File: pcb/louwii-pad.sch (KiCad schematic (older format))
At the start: 50 parts, among them J1 USB_B_Micro, J2 ICSP, J3 IIC, K1 KEYSW, K2 KEYSW, K3 KEYSW, K4 KEYSW, K5 KEYSW, K6 KEYSW, K7 KEYSW, K8 KEYSW, SW1 SW_Push, SW6 Rotary_Encoder_Switch, U1 ATmega32U4-atmel, X1 Crystal

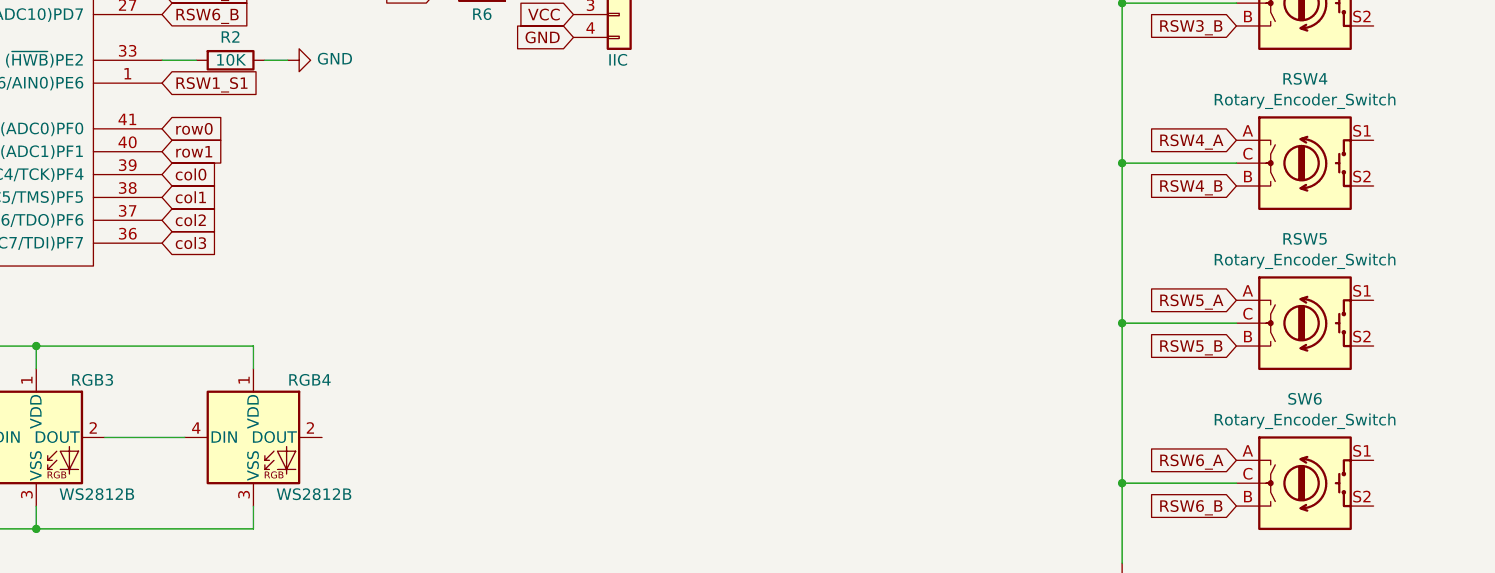
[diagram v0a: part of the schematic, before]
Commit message: finish up schematics and start PCB design
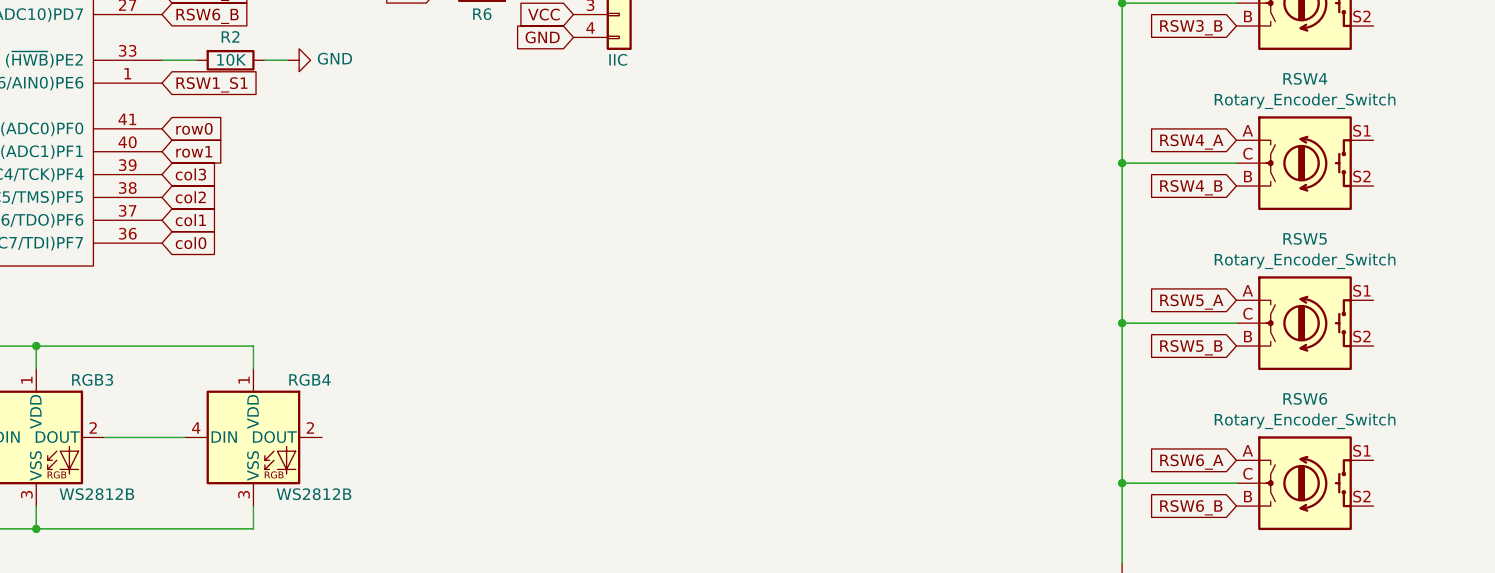
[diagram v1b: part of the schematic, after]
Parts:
- D1, D2, D3, D4, D5, D6, D7, D8: footprint (none) -> Diode_THT:D_DO-35_SOD27_P7.62mm_Horizontal
- J1: footprint (none) -> Connector_USB:USB_Micro-B_Wuerth_629105150521
- J2: footprint (none) -> Connector_PinHeader_2.54mm:PinHeader_2x03_P2.54mm_Vertical
- J3: footprint (none) -> Connector_PinHeader_2.54mm:PinHeader_1x04_P2.54mm_Vertical
- K1, K2, K3, K4, K5, K6, K7, K8: footprint (none) -> Louwii-pad:MX_PCB_100H
- R1, R2, R3, R4, R5, R6: footprint (none) -> Resistor_THT:R_Axial_DIN0207_L6.3mm_D2.5mm_P10.16mm_Horizontal
- RSW1, RSW2, RSW3, RSW4, RSW5: footprint (none) -> Rotary_Encoder:RotaryEncoder_Alps_EC11E-Switch_Vertical_H20mm
- RSW6: renamed from SW6; footprint (none) -> Rotary_Encoder:RotaryEncoder_Alps_EC11E-Switch_Vertical_H20mm
- U1: footprint (none) -> Package_QFP:TQFP-44_10x10mm_P0.8mm
- X1: footprint (none) -> Crystal:Crystal_HC49-U_Vertical
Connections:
- net col0: now also U1.36 ((ADC7/TDI)PF7); no longer U1.39 ((ADC4/TCK)PF4)
- net col1: now also U1.37 ((ADC6/TDO)PF6); no longer U1.38 ((ADC5/TMS)PF5)
- net col2: now also U1.38 ((ADC5/TMS)PF5); no longer U1.37 ((ADC6/TDO)PF6)
- net col3: now also U1.39 ((ADC4/TCK)PF4); no longer U1.36 ((ADC7/TDI)PF7)
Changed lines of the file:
@@
 F 0 "X1" V 1850 3600 50  0000 L CNN
 F 1 "Crystal" V 2250 3500 50  0000 L CNN
-F 2 "" H 2050 3650 50  0001 C CNN
+F 2 "Crystal:Crystal_HC49-U_Vertical" H 2050 3650 50  0001 C CNN
 F 3 "~" H 2050 3650 50  0001 C CNN
 	1    2050 3650
@@
 F 0 "J1" H 7457 1667 50  0000 C CNN
 F 1 "USB_B_Micro" H 7457 1576 50  0000 C CNN
-F 2 "" H 7550 1150 50  0001 C CNN
+F 2 "Connector_USB:USB_Micro-B_Wuerth_629105150521" H 7550 1150 50  0001 C CNN
 F 3 "~" H 7550 1150 50  0001 C CNN
 	1    7400 1200
@@
 F 0 "R3" V 7900 1200 50  0000 C CNN
 F 1 "22" V 8000 1200 50  0000 C CNN
-F 2 "" V 7930 1200 50  0001 C CNN
+F 2 "Resistor_THT:R_Axial_DIN0207_L6.3mm_D2.5mm_P10.16mm_Horizontal" V 7930 1200 50  0001 C CNN
 F 3 "~" H 8000 1200 50  0001 C CNN
 	1    8000 1200
@@
 F 0 "R4" V 8100 1300 50  0000 C CNN
 F 1 "22" V 8000 1300 50  0000 C CNN
-F 2 "" V 7930 1300 50  0001 C CNN
+F 2 "Resistor_THT:R_Axial_DIN0207_L6.3mm_D2.5mm_P10.16mm_Horizontal" V 7930 1300 50  0001 C CNN
 F 3 "~" H 8000 1300 50  0001 C CNN
 	1    8000 1300
@@
 F 0 "R2" V 5250 3600 50  0000 C CNN
 F 1 "10K" V 5350 3600 50  0000 C CNN
-F 2 "" V 5280 3600 50  0001 C CNN
+F 2 "Resistor_THT:R_Axial_DIN0207_L6.3mm_D2.5mm_P10.16mm_Horizontal" V 5280 3600 50  0001 C CNN
 F 3 "~" H 5350 3600 50  0001 C CNN
 	1    5350 3600
@@
 F 0 "R1" V 1900 3200 50  0000 R CNN
 F 1 "10K" V 2000 3300 50  0000 R CNN
-F 2 "" V 1930 3200 50  0001 C CNN
+F 2 "Resistor_THT:R_Axial_DIN0207_L6.3mm_D2.5mm_P10.16mm_Horizontal" V 1930 3200 50  0001 C CNN
 F 3 "~" H 2000 3200 50  0001 C CNN
 	1    2000 3200
@@
 F 0 "RSW1" H 10050 2317 50  0000 C CNN
 F 1 "Rotary_Encoder_Switch" H 10050 2226 50  0000 C CNN
-F 2 "" H 9900 2110 50  0001 C CNN
+F 2 "Rotary_Encoder:RotaryEncoder_Alps_EC11E-Switch_Vertical_H20mm" H 9900 2110 50  0001 C CNN
 F 3 "~" H 10050 2210 50  0001 C CNN
 	1    10050 1950
@@
 F 0 "RSW2" H 10050 3017 50  0000 C CNN
 F 1 "Rotary_Encoder_Switch" H 10050 2926 50  0000 C CNN
-F 2 "" H 9900 2810 50  0001 C CNN
+F 2 "Rotary_Encoder:RotaryEncoder_Alps_EC11E-Switch_Vertical_H20mm" H 9900 2810 50  0001 C CNN
 F 3 "~" H 10050 2910 50  0001 C CNN
 	1    10050 2650
@@
 F 0 "RSW3" H 10050 3717 50  0000 C CNN
 F 1 "Rotary_Encoder_Switch" H 10050 3626 50  0000 C CNN
-F 2 "" H 9900 3510 50  0001 C CNN
+F 2 "Rotary_Encoder:RotaryEncoder_Alps_EC11E-Switch_Vertical_H20mm" H 9900 3510 50  0001 C CNN
 F 3 "~" H 10050 3610 50  0001 C CNN
 	1    10050 3350
@@
 F 0 "RSW4" H 10050 4417 50  0000 C CNN
 F 1 "Rotary_Encoder_Switch" H 10050 4326 50  0000 C CNN
-F 2 "" H 9900 4210 50  0001 C CNN
+F 2 "Rotary_Encoder:RotaryEncoder_Alps_EC11E-Switch_Vertical_H20mm" H 9900 4210 50  0001 C CNN
 F 3 "~" H 10050 4310 50  0001 C CNN
 	1    10050 4050
@@
 F 0 "RSW5" H 10050 5117 50  0000 C CNN
 F 1 "Rotary_Encoder_Switch" H 10050 5026 50  0000 C CNN
-F 2 "" H 9900 4910 50  0001 C CNN
+F 2 "Rotary_Encoder:RotaryEncoder_Alps_EC11E-Switch_Vertical_H20mm" H 9900 4910 50  0001 C CNN
 F 3 "~" H 10050 5010 50  0001 C CNN
 	1    10050 4750
@@
 Connection ~ 9250 4750
 $Comp
-L Device:Rotary_Encoder_Switch SW6
+L Device:Rotary_Encoder_Switch RSW6
 U 1 1 5DB84B4C
 P 10050 5450
-F 0 "SW6" H 10050 5817 50  0000 C CNN
+F 0 "RSW6" H 10050 5817 50  0000 C CNN
 F 1 "Rotary_Encoder_Switch" H 10050 5726 50  0000 C CNN
-F 2 "" H 9900 5610 50  0001 C CNN
+F 2 "Rotary_Encoder:RotaryEncoder_Alps_EC11E-Switch_Vertical_H20mm" H 9900 5610 50  0001 C CNN
 F 3 "~" H 10050 5710 50  0001 C CNN
 	1    10050 5450
@@
 F 0 "K1" H 1700 6450 60  0000 C CNN
 F 1 "KEYSW" H 1700 6350 60  0001 C CNN
-F 2 "" H 1700 6450 60  0000 C CNN
+F 2 "Louwii-pad:MX_PCB_100H" H 1700 6450 60  0001 C CNN
 F 3 "" H 1700 6450 60  0000 C CNN
 	1    1700 6450
@@
 F 0 "D1" V 1346 6571 50  0000 R CNN
 F 1 "D" V 1255 6571 50  0000 R CNN
-F 2 "" H 1300 6650 50  0001 C CNN
+F 2 "Diode_THT:D_DO-35_SOD27_P7.62mm_Horizontal" H 1300 6650 50  0001 C CNN
 F 3 "~" H 1300 6650 50  0001 C CNN
 	1    1300 6650
@@
 F 0 "K2" H 1700 7050 60  0000 C CNN
 F 1 "KEYSW" H 1700 6950 60  0001 C CNN
-F 2 "" H 1700 7050 60  0000 C CNN
+F 2 "Louwii-pad:MX_PCB_100H" H 1700 7050 60  0001 C CNN
 F 3 "" H 1700 7050 60  0000 C CNN
 	1    1700 7050
@@
 F 0 "D2" V 1346 7171 50  0000 R CNN
 F 1 "D" V 1255 7171 50  0000 R CNN
-F 2 "" H 1300 7250 50  0001 C CNN
+F 2 "Diode_THT:D_DO-35_SOD27_P7.62mm_Horizontal" H 1300 7250 50  0001 C CNN
 F 3 "~" H 1300 7250 50  0001 C CNN
 	1    1300 7250
@@
 F 0 "K3" H 2600 6450 60  0000 C CNN
 F 1 "KEYSW" H 2600 6350 60  0001 C CNN
-F 2 "" H 2600 6450 60  0000 C CNN
+F 2 "Louwii-pad:MX_PCB_100H" H 2600 6450 60  0001 C CNN
 F 3 "" H 2600 6450 60  0000 C CNN
 	1    2600 6450
@@
 F 0 "D3" V 2246 6571 50  0000 R CNN
 F 1 "D" V 2155 6571 50  0000 R CNN
-F 2 "" H 2200 6650 50  0001 C CNN
+F 2 "Diode_THT:D_DO-35_SOD27_P7.62mm_Horizontal" H 2200 6650 50  0001 C CNN
 F 3 "~" H 2200 6650 50  0001 C CNN
 	1    2200 6650
@@
 F 0 "K4" H 2600 7050 60  0000 C CNN
 F 1 "KEYSW" H 2600 6950 60  0001 C CNN
-F 2 "" H 2600 7050 60  0000 C CNN
+F 2 "Louwii-pad:MX_PCB_100H" H 2600 7050 60  0001 C CNN
 F 3 "" H 2600 7050 60  0000 C CNN
 	1    2600 7050
@@
 F 0 "D4" V 2246 7171 50  0000 R CNN
 F 1 "D" V 2155 7171 50  0000 R CNN
-F 2 "" H 2200 7250 50  0001 C CNN
+F 2 "Diode_THT:D_DO-35_SOD27_P7.62mm_Horizontal" H 2200 7250 50  0001 C CNN
 F 3 "~" H 2200 7250 50  0001 C CNN
 	1    2200 7250
@@
 F 0 "K5" H 3500 6450 60  0000 C CNN
 F 1 "KEYSW" H 3500 6350 60  0001 C CNN
-F 2 "" H 3500 6450 60  0000 C CNN
+F 2 "Louwii-pad:MX_PCB_100H" H 3500 6450 60  0001 C CNN
 F 3 "" H 3500 6450 60  0000 C CNN
 	1    3500 6450
@@
 F 0 "D5" V 3146 6571 50  0000 R CNN
 F 1 "D" V 3055 6571 50  0000 R CNN
-F 2 "" H 3100 6650 50  0001 C CNN
+F 2 "Diode_THT:D_DO-35_SOD27_P7.62mm_Horizontal" H 3100 6650 50  0001 C CNN
 F 3 "~" H 3100 6650 50  0001 C CNN
 	1    3100 6650
@@
 F 0 "K6" H 3500 7050 60  0000 C CNN
 F 1 "KEYSW" H 3500 6950 60  0001 C CNN
-F 2 "" H 3500 7050 60  0000 C CNN
+F 2 "Louwii-pad:MX_PCB_100H" H 3500 7050 60  0001 C CNN
 F 3 "" H 3500 7050 60  0000 C CNN
 	1    3500 7050
@@
 F 0 "D6" V 3146 7171 50  0000 R CNN
 F 1 "D" V 3055 7171 50  0000 R CNN
-F 2 "" H 3100 7250 50  0001 C CNN
+F 2 "Diode_THT:D_DO-35_SOD27_P7.62mm_Horizontal" H 3100 7250 50  0001 C CNN
 F 3 "~" H 3100 7250 50  0001 C CNN
 	1    3100 7250
@@
 F 0 "K7" H 4400 6450 60  0000 C CNN
 F 1 "KEYSW" H 4400 6350 60  0001 C CNN
-F 2 "" H 4400 6450 60  0000 C CNN
+F 2 "Louwii-pad:MX_PCB_100H" H 4400 6450 60  0001 C CNN
 F 3 "" H 4400 6450 60  0000 C CNN
 	1    4400 6450
@@
 F 0 "D7" V 4046 6571 50  0000 R CNN
 F 1 "D" V 3955 6571 50  0000 R CNN
-F 2 "" H 4000 6650 50  0001 C CNN
+F 2 "Diode_THT:D_DO-35_SOD27_P7.62mm_Horizontal" H 4000 6650 50  0001 C CNN
 F 3 "~" H 4000 6650 50  0001 C CNN
 	1    4000 6650
@@
 F 0 "K8" H 4400 7050 60  0000 C CNN
 F 1 "KEYSW" H 4400 6950 60  0001 C CNN
-F 2 "" H 4400 7050 60  0000 C CNN
+F 2 "Louwii-pad:MX_PCB_100H" H 4400 7050 60  0001 C CNN
 F 3 "" H 4400 7050 60  0000 C CNN
 	1    4400 7050
@@
 F 0 "D8" V 4046 7171 50  0000 R CNN
 F 1 "D" V 3955 7171 50  0000 R CNN
-F 2 "" H 4000 7250 50  0001 C CNN
+F 2 "Diode_THT:D_DO-35_SOD27_P7.62mm_Horizontal" H 4000 7250 50  0001 C CNN
 F 3 "~" H 4000 7250 50  0001 C CNN
 	1    4000 7250
@@
 Text GLabel 5050 4000 2    50   Input ~ 0
 row1
+Text GLabel 5050 4400 2    50   Input ~ 0
+col0
+Text GLabel 5050 4200 2    50   Input ~ 0
+col2
+Text GLabel 5050 4300 2    50   Input ~ 0
+col1
 Text GLabel 5050 4100 2    50   Input ~ 0
-col0
-Text GLabel 5050 4300 2    50   Input ~ 0
-col2
-Text GLabel 5050 4200 2    50   Input ~ 0
-col1
-Text GLabel 5050 4400 2    50   Input ~ 0
 col3
 Text GLabel 5050 2700 2    50   Input ~ 0
@@
 F 0 "U1" H 3825 4865 50  0000 C CNN
 F 1 "ATmega32U4-atmel" H 3825 4774 50  0000 C CNN
-F 2 "" H 5050 4150 50  0001 C CNN
+F 2 "Package_QFP:TQFP-44_10x10mm_P0.8mm" H 5050 4150 50  0001 C CNN
 F 3 "" H 5050 4150 50  0001 C CNN
 	1    3850 3050
@@
 F 0 "J2" H 7000 2900 50  0000 C CNN
 F 1 "ICSP" H 7000 2500 50  0000 C CNN
-F 2 "" H 6950 2700 50  0001 C CNN
+F 2 "Connector_PinHeader_2.54mm:PinHeader_2x03_P2.54mm_Vertical" H 6950 2700 50  0001 C CNN
 F 3 "~" H 6950 2700 50  0001 C CNN
 	1    6950 2700
@@
 F 0 "J3" H 7000 3500 50  0000 L CNN
 F 1 "IIC" H 7000 3000 50  0000 L CNN
-F 2 "" H 7050 3300 50  0001 C CNN
+F 2 "Connector_PinHeader_2.54mm:PinHeader_1x04_P2.54mm_Vertical" H 7050 3300 50  0001 C CNN
 F 3 "~" H 7050 3300 50  0001 C CNN
 	1    7050 3300
@@
 F 0 "R5" V 6750 3200 50  0000 C CNN
 F 1 "4.7k" V 6650 3200 50  0000 C CNN
-F 2 "" V 6580 3200 50  0001 C CNN
+F 2 "Resistor_THT:R_Axial_DIN0207_L6.3mm_D2.5mm_P10.16mm_Horizontal" V 6580 3200 50  0001 C CNN
 F 3 "~" H 6650 3200 50  0001 C CNN
 	1    6650 3200
@@
 F 0 "R6" V 6350 3300 50  0000 C CNN
 F 1 "4.7k" V 6450 3300 50  0000 C CNN
-F 2 "" V 6380 3300 50  0001 C CNN
+F 2 "Resistor_THT:R_Axial_DIN0207_L6.3mm_D2.5mm_P10.16mm_Horizontal" V 6380 3300 50  0001 C CNN
 F 3 "~" H 6450 3300 50  0001 C CNN
 	1    6450 3300
